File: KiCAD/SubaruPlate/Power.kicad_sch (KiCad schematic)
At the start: 1 part

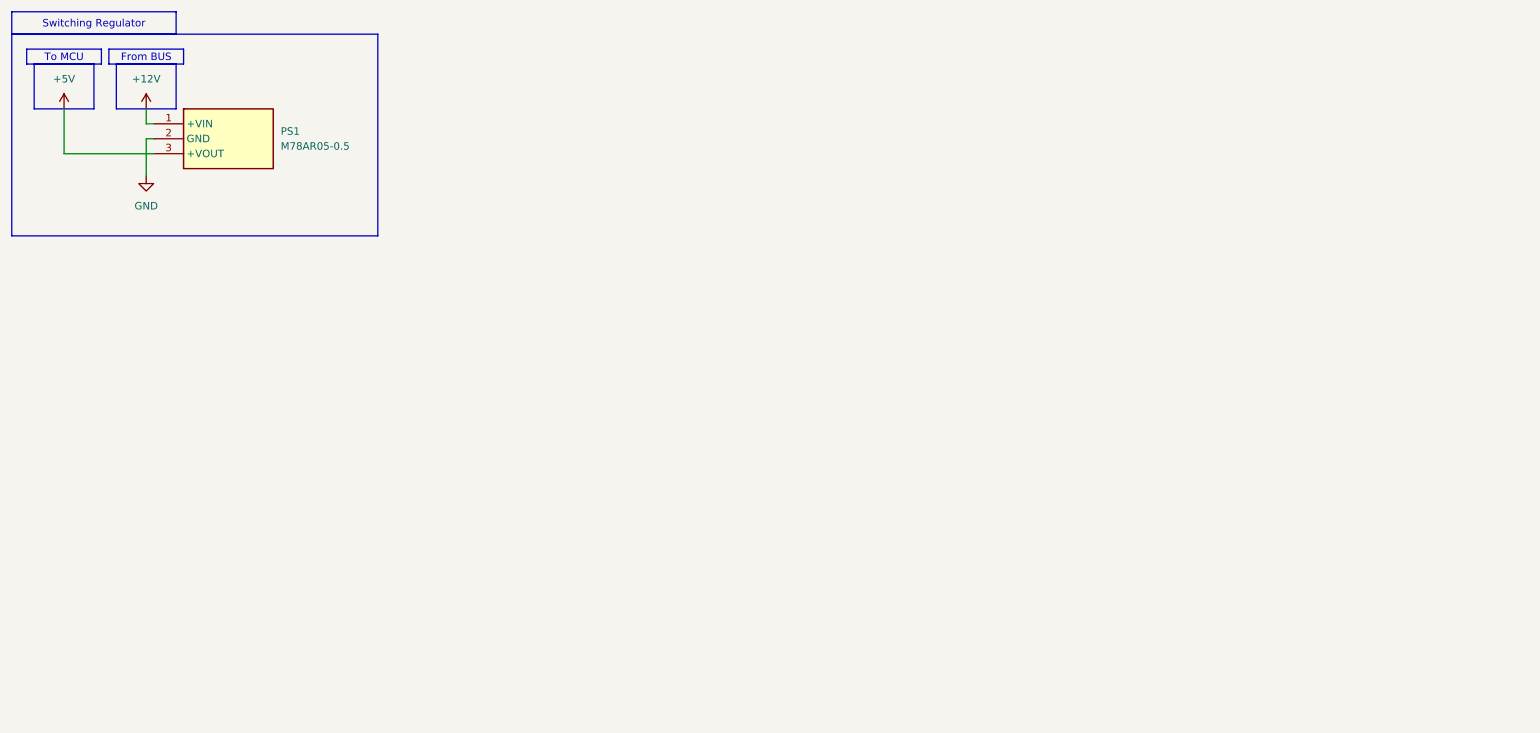
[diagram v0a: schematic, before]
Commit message: 後は最終確認
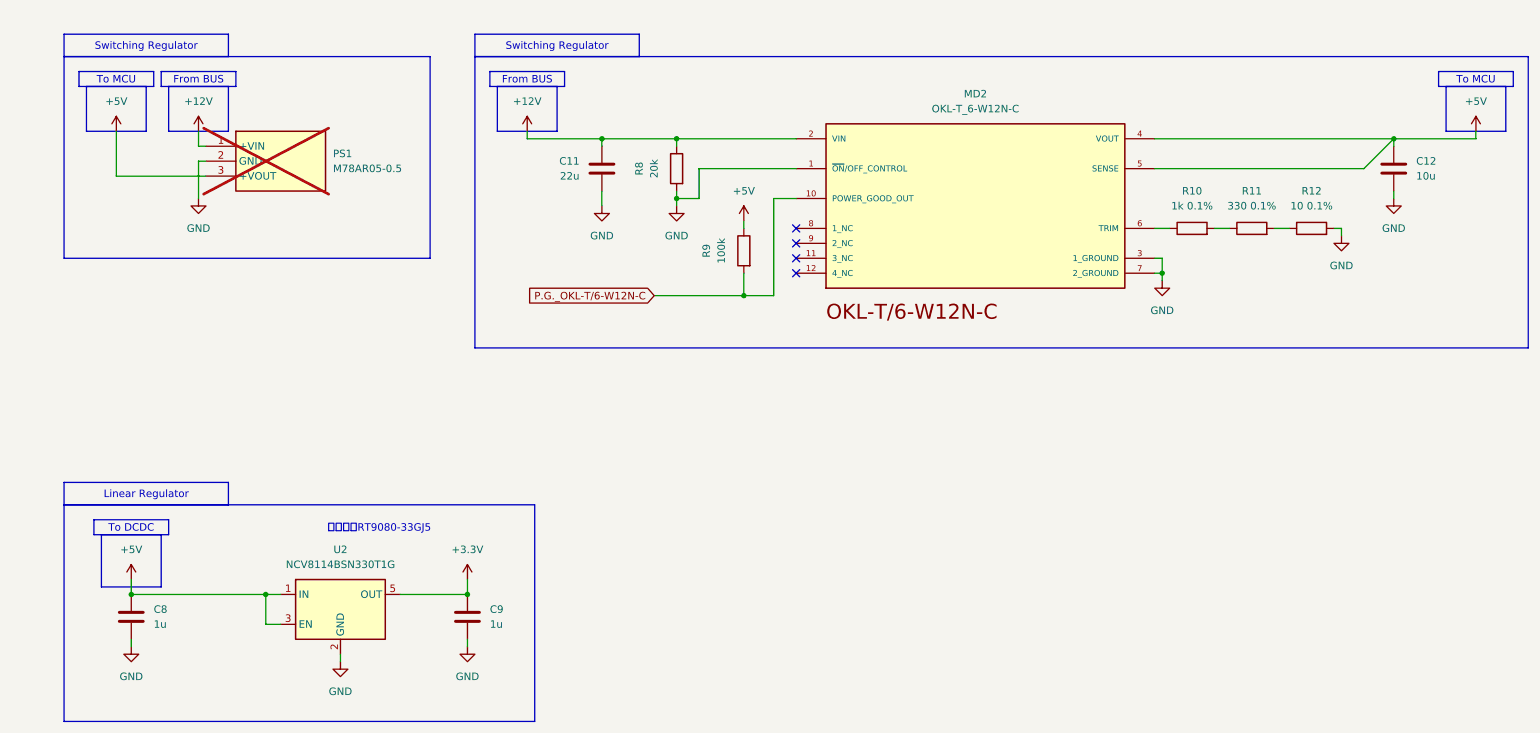
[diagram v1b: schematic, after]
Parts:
- added C11: 22u, Capacitor_SMD:C_0805_2012Metric_Pad1.18x1.45mm_HandSolder, symbol Device:C
- added C12: 10u, Capacitor_SMD:C_0805_2012Metric_Pad1.18x1.45mm_HandSolder, symbol Device:C
- added C8, C9: 1u, Capacitor_SMD:C_0603_1608Metric_Pad1.08x0.95mm_HandSolder, symbol Device:C
- added MD2: OKL-T_6-W12N-C, TSRP_IC:MURATA_OKL-T-6-W12N-C_0, symbol TSRP_IC:OKL-T_6-W12N-C
- added R10: 1k 0.1%, Resistor_SMD:R_0603_1608Metric_Pad0.98x0.95mm_HandSolder, symbol Device:R
- added R11: 330 0.1%, Resistor_SMD:R_0603_1608Metric_Pad0.98x0.95mm_HandSolder, symbol Device:R
- added R12: 10 0.1%, Resistor_SMD:R_0603_1608Metric_Pad0.98x0.95mm_HandSolder, symbol Device:R
- added R8: 20k, Resistor_SMD:R_0603_1608Metric_Pad0.98x0.95mm_HandSolder, symbol Device:R
- added R9: 100k, Resistor_SMD:R_0603_1608Metric_Pad0.98x0.95mm_HandSolder, symbol Device:R
- added U2: NCV8114BSN330T1G, Package_TO_SOT_SMD:TSOT-23-5, symbol Regulator_Linear:NCV8114BSN330T1G
- PS1: now not fitted; now left out of the parts list
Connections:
- net +12V: now also C11.1, MD2.2 (VIN), R8.1
- net +5V: now also C12.1, C8.1, MD2.4 (VOUT), MD2.5 (SENSE), R9.1, U2.1 (IN), U2.3 (EN)
- net GND: now also C11.2, C12.2, C8.2, C9.2, MD2.1 (~{ON}/OFF_CONTROL), MD2.3 (1_GROUND), MD2.7 (2_GROUND), R12.2, R8.2, U2.2 (GND)
- new net: R10.2, R11.1
- new net: R11.2, R12.1
- new net: MD2.6 (TRIM), R10.1
- new net +3.3V: C9.1, U2.5 (OUT)
- new net P.G._OKL-T/6-W12N-C: MD2.10 (POWER_GOOD_OUT), R9.2
- no-connect marks 0 -> 4
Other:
- note added: "本当は，RT9080-33GJ5"
